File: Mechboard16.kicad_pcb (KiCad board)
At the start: 2 copper layers, 386.1 x 97 mm, 254 parts, among them CN1 CONN_C16, CN2 CONN_+4, J201 USB_B, J202 CONN_ICSP, J203 CONN_MRESET, J204 CONN_LED, Q201 MMBT3904, Q202 MMBT3904, SW0:0 KEY_DEL, SW0:1 KEY_RET, SW0:2 KEY_PND, SW0:3 KEY_HLP, SW0:4 KEY_F1, SW0:5 KEY_F2, SW0:6 KEY_F3, SW0:7 KEY_AT, SW1:0 KEY_3, SW1:1 KEY_W, SW1:2 KEY_A, SW1:3 KEY_4, SW1:4 KEY_Z, SW1:5 KEY_S, SW1:6 KEY_E, SW1:7 KEY_LSH, SW1B:7 KEY_RSH, SW1C:7 KEY_CLK, SW201 SW_RESET, SW2:0 KEY_5, SW2:1 KEY_R, SW2:2 KEY_D, SW2:3 KEY_6, SW2:4 KEY_C, SW2:5 KEY_F, SW2:6 KEY_T, SW2:7 KEY_X, SW3:0 KEY_7, SW3:1 KEY_Y, SW3:2 KEY_G, SW3:3 KEY_8, SW3:4 KEY_B, SW3:5 KEY_H, SW3:6 KEY_U, SW3:7 KEY_V, SW4:0 KEY_9, SW4:1 KEY_I, SW4:2 KEY_J, SW4:3 KEY_0, SW4:4 KEY_M, SW4:5 KEY_K, SW4:6 KEY_O, SW4:7 KEY_N, SW5:0 KEY_DN, SW5:1 KEY_P, SW5:2 KEY_L, SW5:3 KEY_UP, SW5:4 KEY_DOT, SW5:5 KEY_COL, SW5:6 KEY_MIN, SW5:7 KEY_COM, SW6:0 KEY_LF, SW6:1 KEY_AST, SW6:2 KEY_SEM, SW6:3 KEY_RT, SW6:4 KEY_ESC, SW6:5 KEY_EQ, SW6:6 KEY_PLS, SW6:7 KEY_SLA, SW7:0 KEY_1, SW7:1 KEY_CLR, SW7:2 KEY_CTL, SW7:3 KEY_2, SW7:4 KEY_SPC, SW7:5 KEY_CMD, SW7:6 KEY_Q, SW7:7 KEY_RUN, U1 4066, U2 NE555, U201 ATmega32U4-AU, U202 MAX7221, Y201 16M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

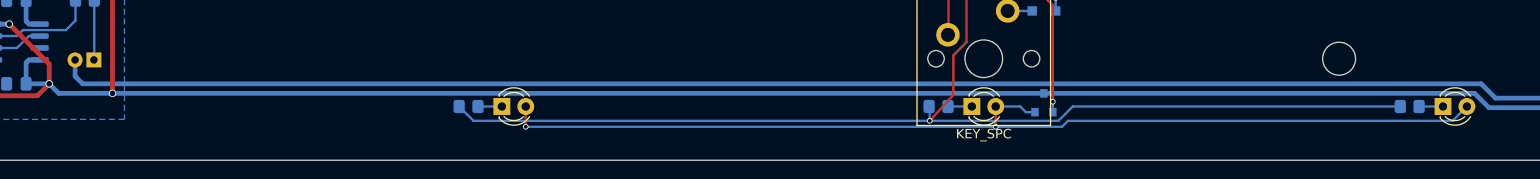
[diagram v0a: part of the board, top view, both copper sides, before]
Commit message: Finaaaaaaaaaal touches
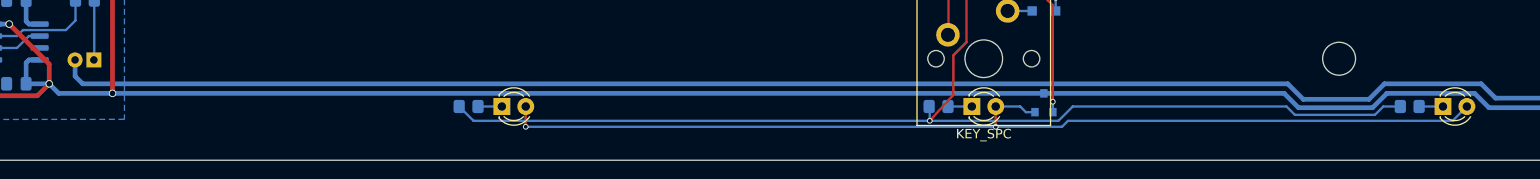
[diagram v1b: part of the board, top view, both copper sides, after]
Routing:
- net GND: track 476.0 -> 477.4 mm
- net +5V: track 649.9 -> 651.1 mm
- net /USB Controller/lcol4: track 590.6 -> 591.4 mm
